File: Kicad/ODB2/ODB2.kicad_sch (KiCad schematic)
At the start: 32 parts, among them U1 STM32F412ZGTx

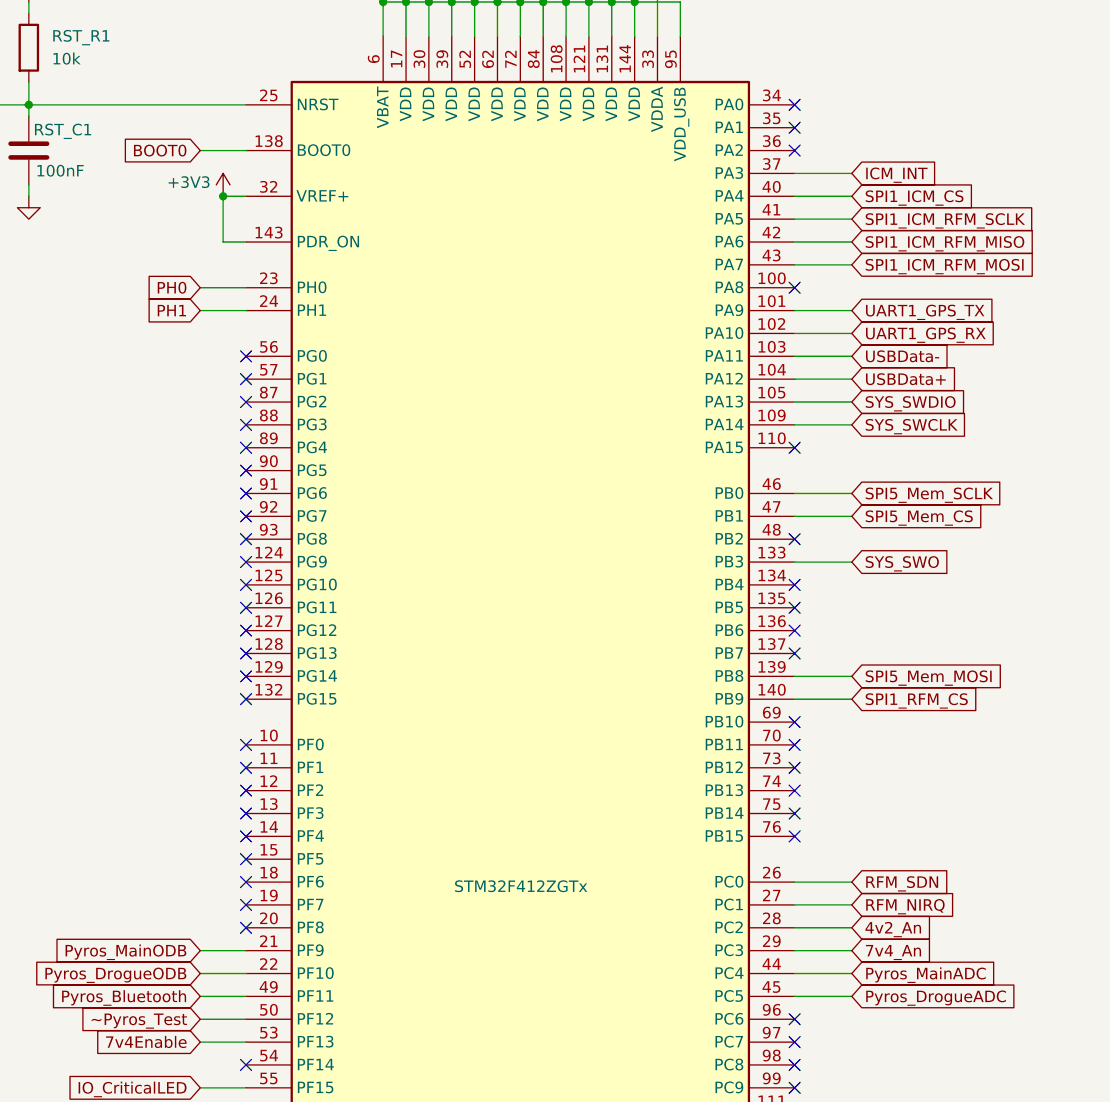
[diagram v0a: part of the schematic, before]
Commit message: Final fixes
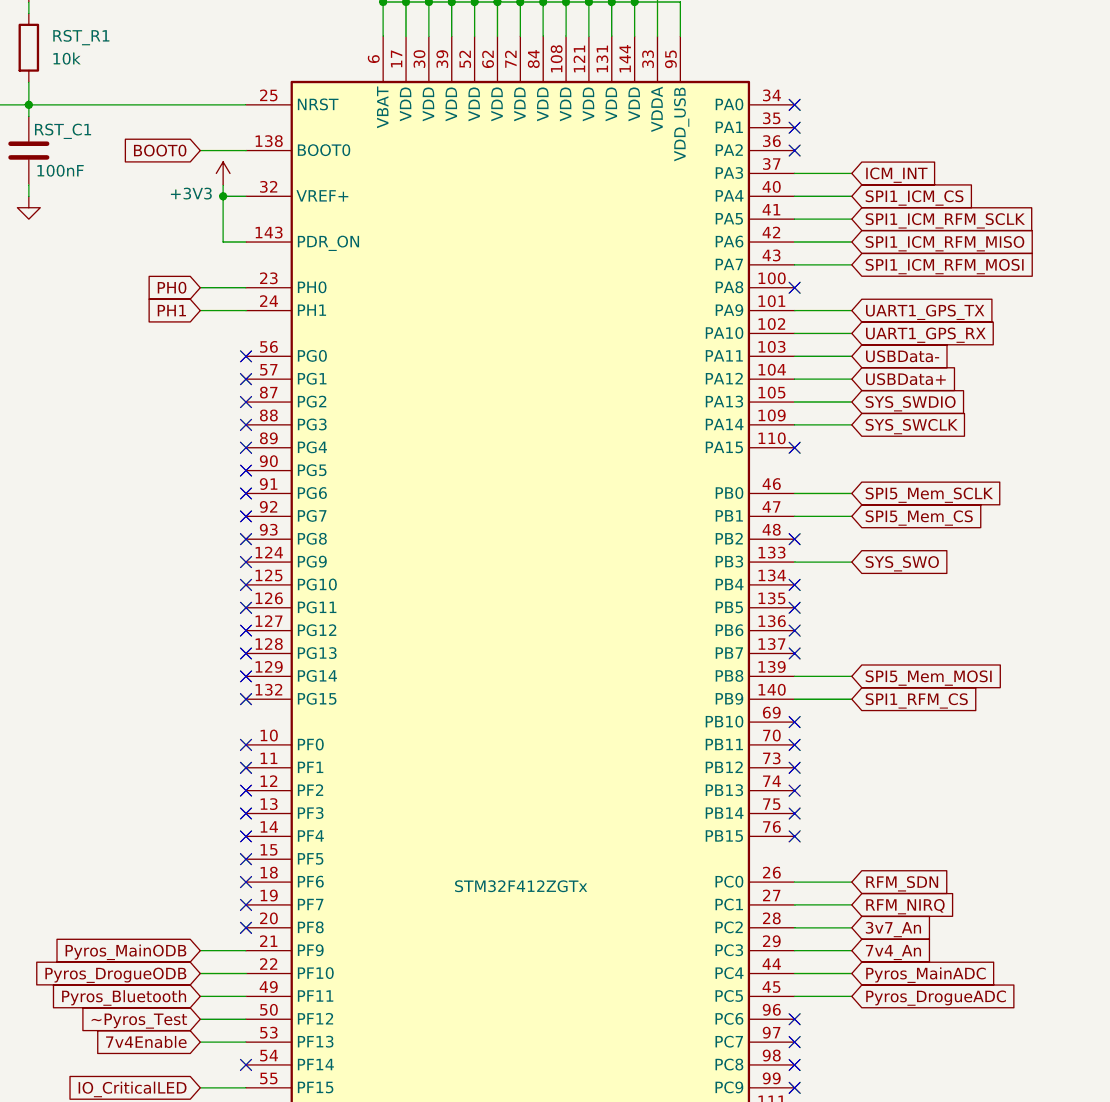
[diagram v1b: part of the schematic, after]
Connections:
- net 4v2_An renamed 3v7_An
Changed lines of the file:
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@@
+	(wire
+		(pts
+			(xy 167.64 64.77) (xy 167.64 66.04)
+		)
+		(stroke
+			(width 0)
+			(type default)
+		)
+	)
 	(wire
 		(pts
@@
 		)
 	)
-	(global_label "4v2_An"
+	(global_label "3v7_An"
 		(shape input)
 		(at 237.49 147.32 0)
@@
 	(symbol
 		(lib_id "power:+3V3")
-		(at 167.64 66.04 0)
+		(at 167.64 64.77 0)
 		(unit 1)
 		(exclude_from_sim no)
@@
 		(dnp no)
 		(property "Reference" "#PWR089"
-			(at 167.64 69.85 0)
+			(at 167.64 68.58 0)
 			(effects
 				(font
@@
 		)
 		(property "Value" "+3V3"
-			(at 163.83 64.516 0)
+			(at 164.084 65.786 0)
 			(effects
 				(font
@@
 		)
 		(property "Footprint" ""
-			(at 167.64 66.04 0)
+			(at 167.64 64.77 0)
 			(effects
 				(font
@@
 		)
 		(property "Datasheet" ""
-			(at 167.64 66.04 0)
+			(at 167.64 64.77 0)
 			(effects
 				(font
@@
 		)
 		(property "Description" "Power symbol creates a global label with name \"+3V3\""
-			(at 167.64 66.04 0)
-			(effects
-				(font
+			(at 167.64 64.77 0)
+			(effects
+				(font
